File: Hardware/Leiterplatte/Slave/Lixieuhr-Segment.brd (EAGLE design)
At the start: 45 x 50 mm, 43 parts, among them U1 APA102C, U10 APA102C, U11 APA102C, U12 APA102C, U13 APA102C, U14 APA102C, U15 APA102C, U16 APA102C, U17 APA102C, U18 APA102C, U19 APA102C, U2 APA102C, U20 APA102C, U3 APA102C, U4 APA102C, U5 APA102C, U6 APA102C, U7 APA102C, U8 APA102C, U9 APA102C

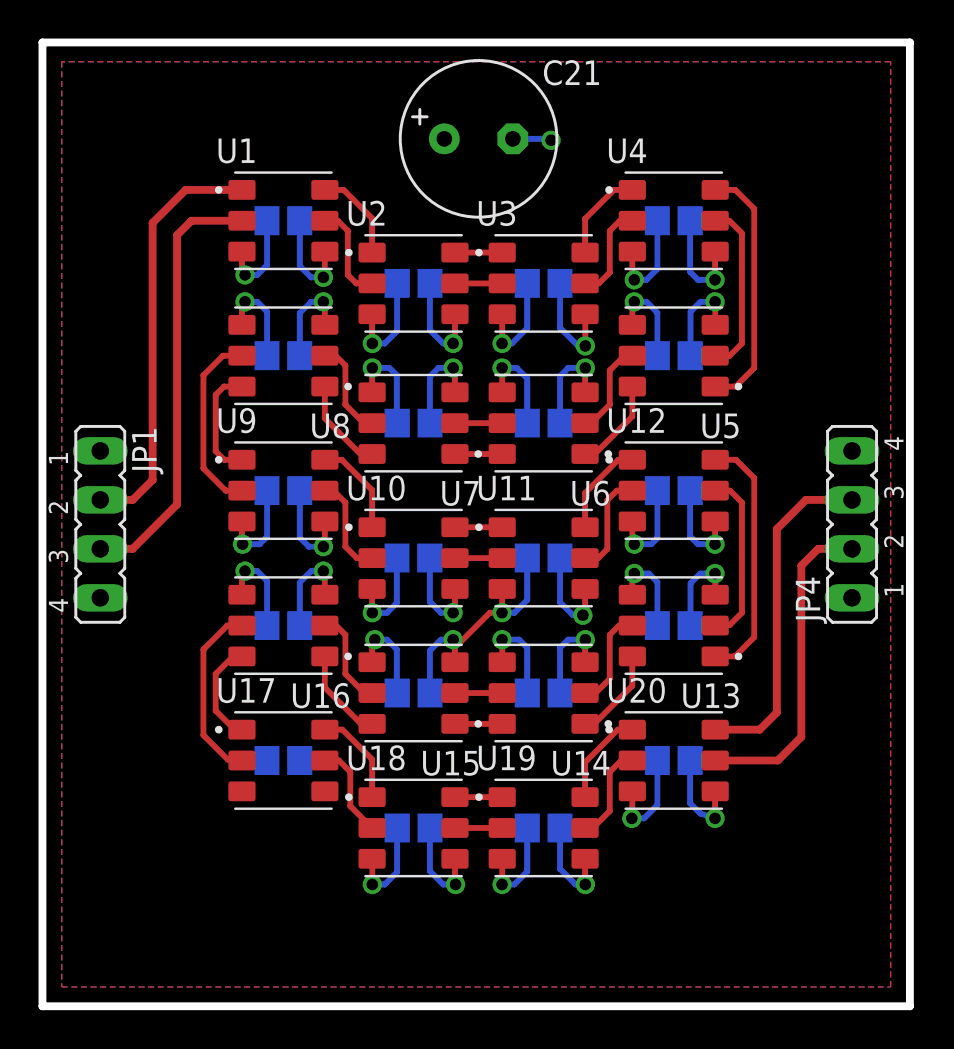
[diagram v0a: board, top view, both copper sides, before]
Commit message: Segmentplatine_V03
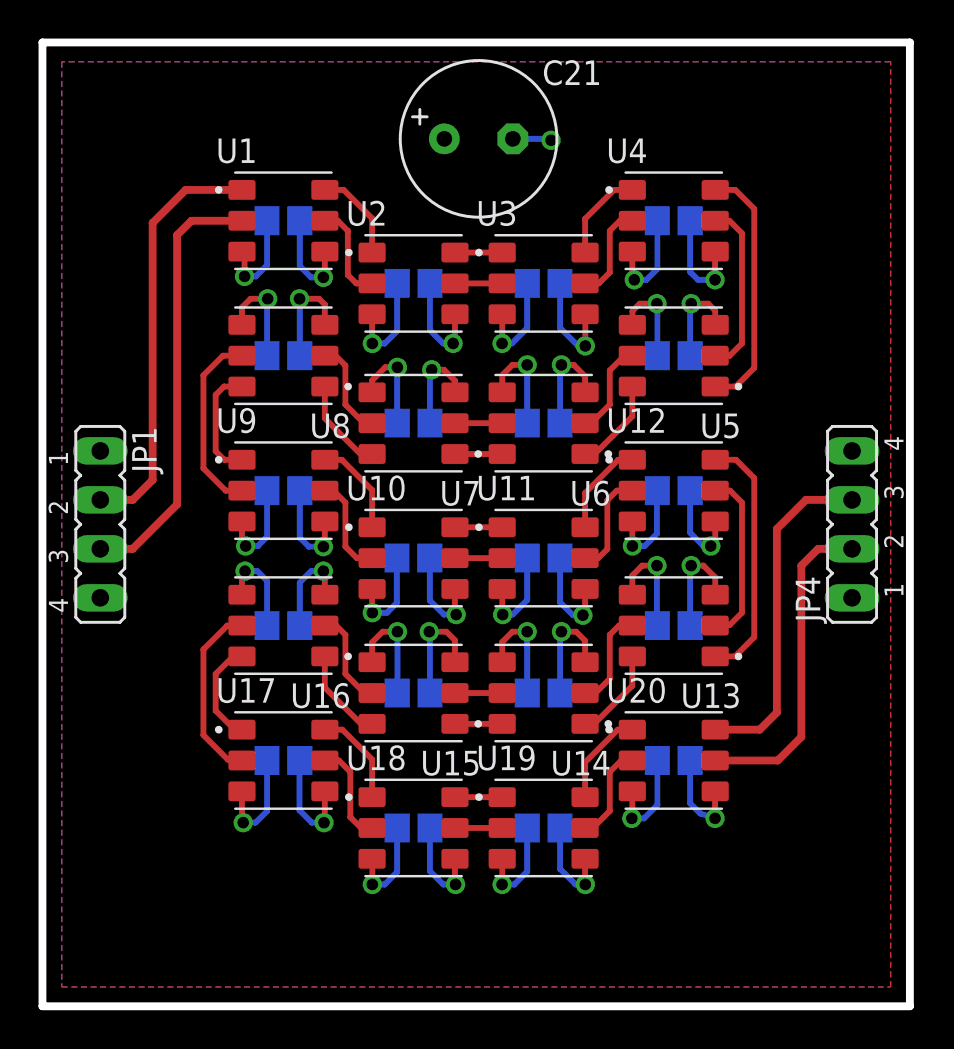
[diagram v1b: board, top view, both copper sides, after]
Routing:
- net V+: track 97.4 -> 106.5 mm, vias 19 -> 20
- net GND: track 102.2 -> 108.1 mm, vias 20 -> 21
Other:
- board text added: "0.60 mm"
- board text added: "0.80 mm"
- board text added: "0.90 mm"
- board text added: "0.91 mm"
- board text added: "2"
- board text added: "41"
- board text added: "51"
- board text added: "8"
- board text added: "Bohrplan"
- board text added: "CNT"
- board text added: "Material: FR4 1,5mm 35u Cu"
- board text added: "SIZE"
- board text added: "SYM"
- board text added: "TOTAL"
- board text added: "Toleranz: Aussenmass -0,5mm, sonst +/_0,2mm"

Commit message: Leiterplatten V05
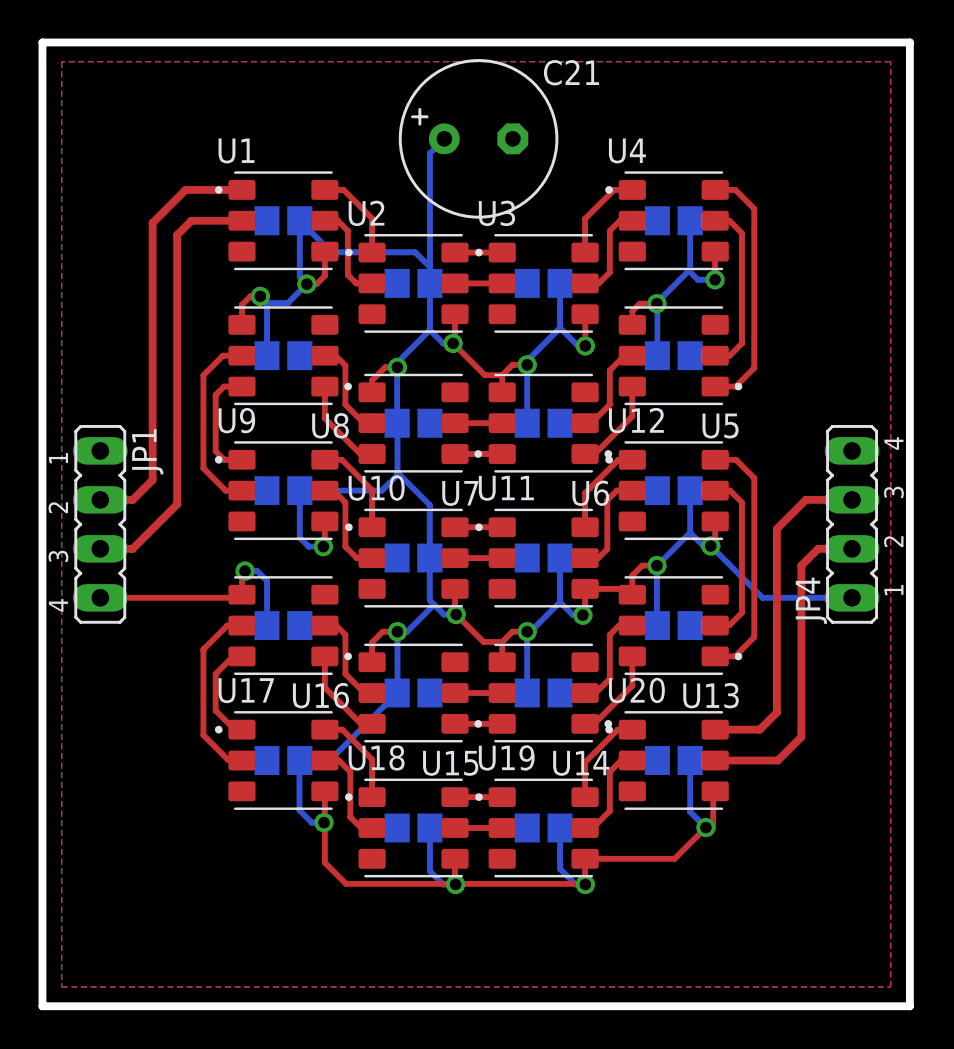
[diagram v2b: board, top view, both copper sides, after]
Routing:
- net GND: track 108.1 -> 0.24 mm, vias 21 -> 0
- net V+: track 106.5 -> 209.8 mm
- added copper zone on layer 16, net GND
- removed copper zone on layer 16, net V+
